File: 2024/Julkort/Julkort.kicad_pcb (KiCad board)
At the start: 2 copper layers, 98.8 x 68 mm, 29 parts, among them J1 SK-3296S-01-L1, U1 ATtiny44A-M, U2 L78L05_SOT89

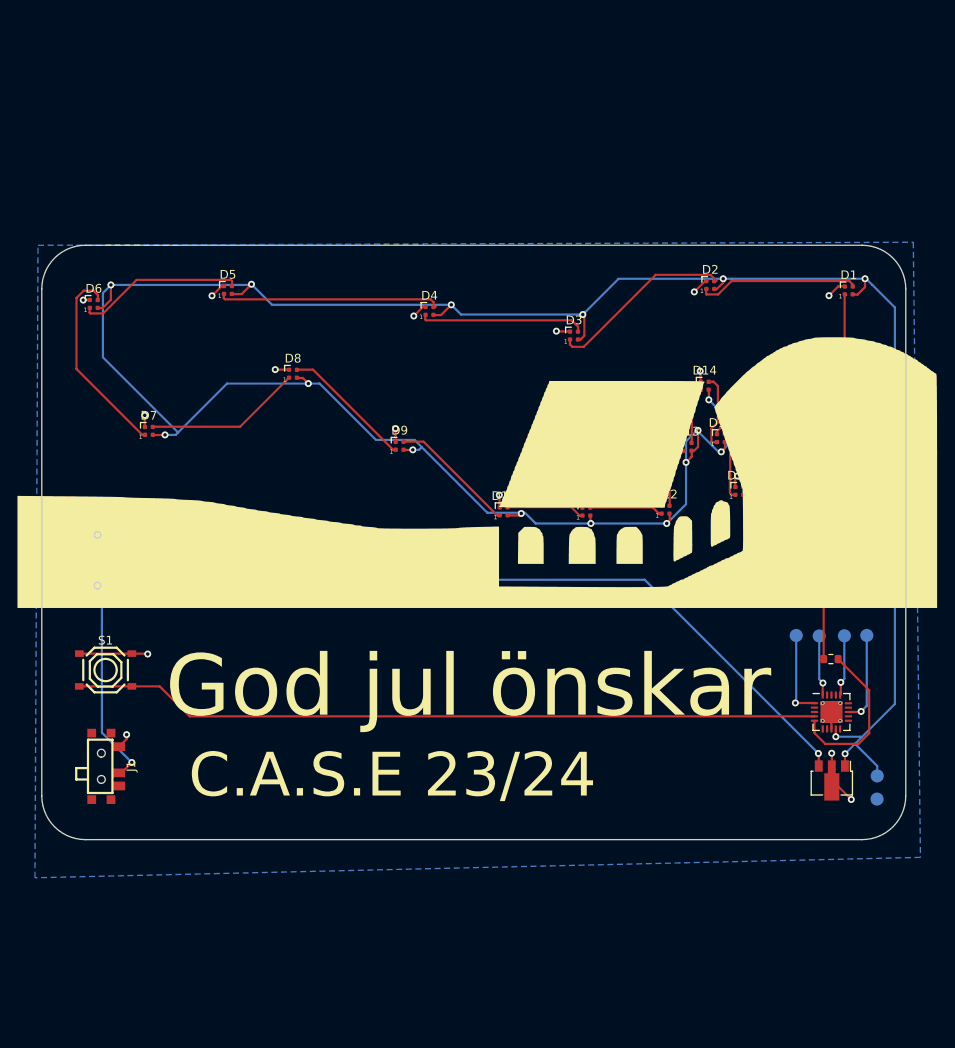
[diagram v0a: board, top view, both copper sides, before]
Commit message: 2024 v1
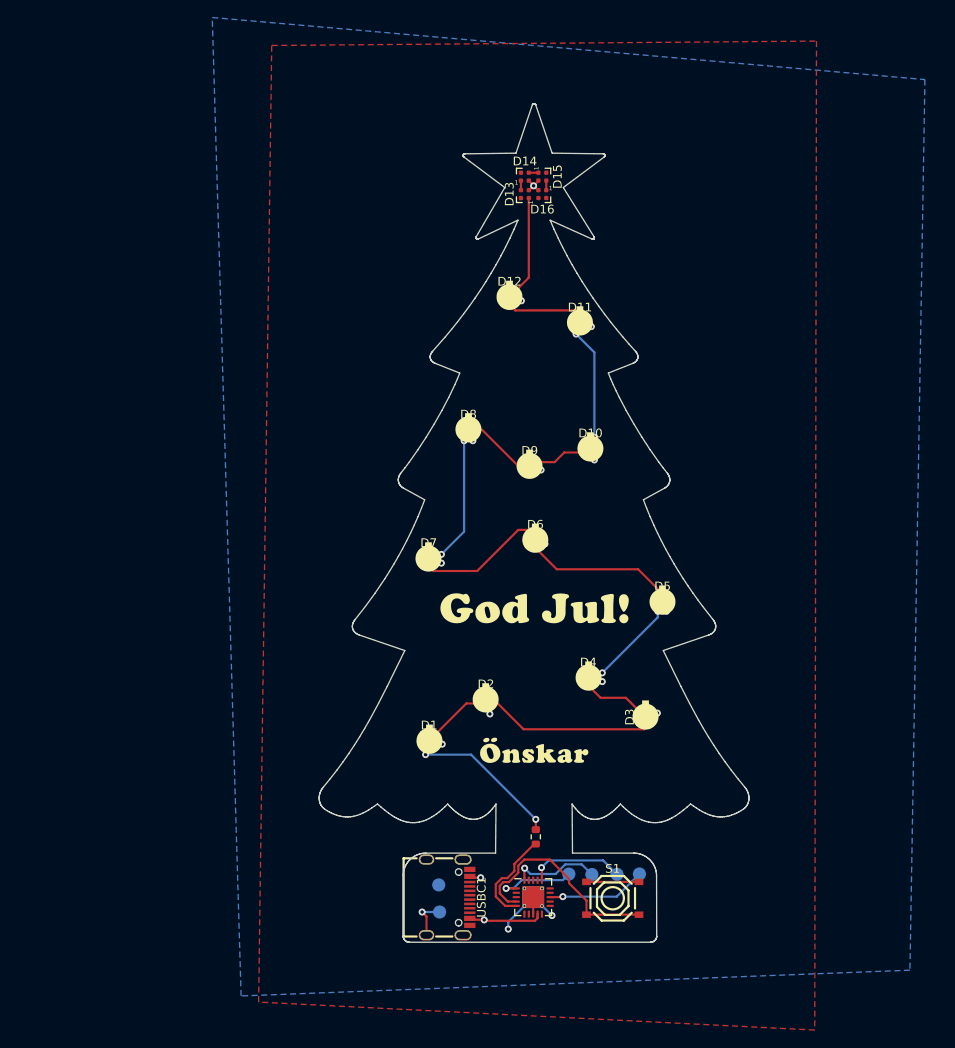
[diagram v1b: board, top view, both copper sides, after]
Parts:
- removed G***: LOGO, gra:wwwwwwwwwwwwwwwwww
- removed J1: SK-3296S-01-L1, ProLib_pcs_2024-11-12:SW-SMD_3P-P1.50_L2.7-W6.6
- removed U2: L78L05_SOT89, Package_TO_SOT_SMD:SOT-89-3
- USBC1: moved to F.Cu
- moved D1 70.4 mm to (117.5, 127.2)
- moved S1 63.6 mm to (138.5, 145.2)
- moved D5 61.2 mm to (144.2, 111.3)
- moved D6 57.3 mm to (129.7, 104.2)
- moved USBC1 56.5 mm to (119.7, 145.1), turned to -90 degrees
- moved D2 53.9 mm to (124.0, 122.5)
- moved TP5 51.7 mm to (118.6, 143.7)
- moved TP6 51.7 mm to (118.7, 146.8)
- moved D4 45.7 mm to (135.7, 120.0)
- moved D3 44.4 mm to (142.2, 124.5), turned to 90 degrees
- moved D16 40.7 mm to (130.4, 64.7), turned to 180 degrees
- moved U1 40.1 mm to (129.4, 145.1)
- moved R1 39.4 mm to (129.7, 138.2), turned to 90 degrees
- moved TP1 37.7 mm to (133.5, 142.5)
- moved TP2 37.7 mm to (136.1, 142.5)
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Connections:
- USBC1 pad 0: Net-(J1-COM) -> GND
- USBC1 pad 1: Net-(J1-COM) -> GND
- USBC1 pad 2: Net-(J1-COM) -> GND
- USBC1 pad 3: Net-(J1-COM) -> GND
- USBC1 pad A1: Net-(J1-COM) -> GND
- USBC1 pad A12: Net-(J1-COM) -> GND
- USBC1 pad A4: Net-(U2-IN) -> VCC_REG
- USBC1 pad A9: Net-(U2-IN) -> VCC_REG
- USBC1 pad B1: Net-(J1-COM) -> GND
- USBC1 pad B12: Net-(J1-COM) -> GND
- USBC1 pad B4: Net-(U2-IN) -> VCC_REG
- USBC1 pad B9: Net-(U2-IN) -> VCC_REG
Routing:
- net VCC_REG: track 310.5 -> 23.8 mm, vias 19 -> 15
- net Net-(U2-IN): track 96.3 -> 0.00 mm, vias 1 -> 0
- net Net-(U1-PA1): track 85.5 -> 24.6 mm
- net Net-(J1-COM): track 42.9 -> 0.00 mm, vias 1 -> 0
- net Net-(D1-DIN): track 42.7 -> 18.0 mm, vias 0 -> 2
- net GND: track 41.0 -> 17.8 mm, vias 20 -> 3
- net Net-(D4-DOUT): track 25.4 -> 11.6 mm, vias 0 -> 2
- net Net-(D1-DOUT): track 18.4 -> 7.17 mm
- net Net-(D3-DOUT): track 18.9 -> 7.99 mm
- net Net-(D10-DIN): track 14.4 -> 6.51 mm
- net Net-(U1-AREF/PA0): track 18.6 -> 11.1 mm
- net Net-(D14-DOUT): track 8.53 -> 1.10 mm
- net Net-(D8-DOUT): track 15.0 -> 8.19 mm
- net Net-(D15-DOUT): track 7.84 -> 1.10 mm
- net Net-(D6-DOUT): track 22.6 -> 16.0 mm
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- added copper zone on F.Cu, net GND
- added copper zone on B.Cu, net VCC_REG
- removed copper zone on B.Cu, net GND
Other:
- board size 98.8 x 68 mm -> 49.1 x 95.9 mm
- board text removed: "C.A.S.E 23/24"
- board text removed: "God jul önskar"
